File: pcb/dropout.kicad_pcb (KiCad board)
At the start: 2 copper layers, 228.6 x 94.4 mm, 64 parts, among them J1 Conn_01x04_Male, SW1 Rotary_Encoder_Switch, SW2 SW_Push, U1 ProMicro, U2 ProMicro

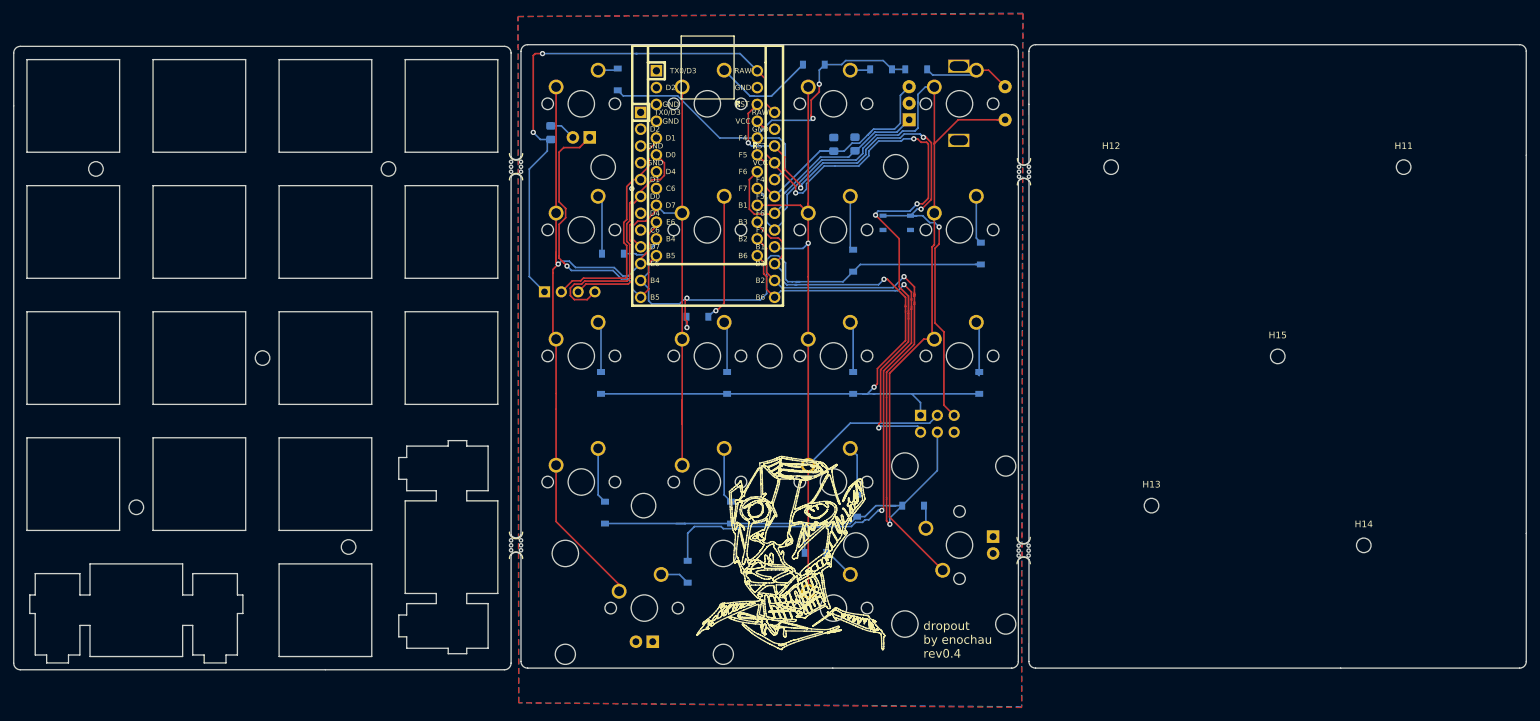
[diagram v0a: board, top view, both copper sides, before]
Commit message: updating to rev0.5
updating to rev0.5
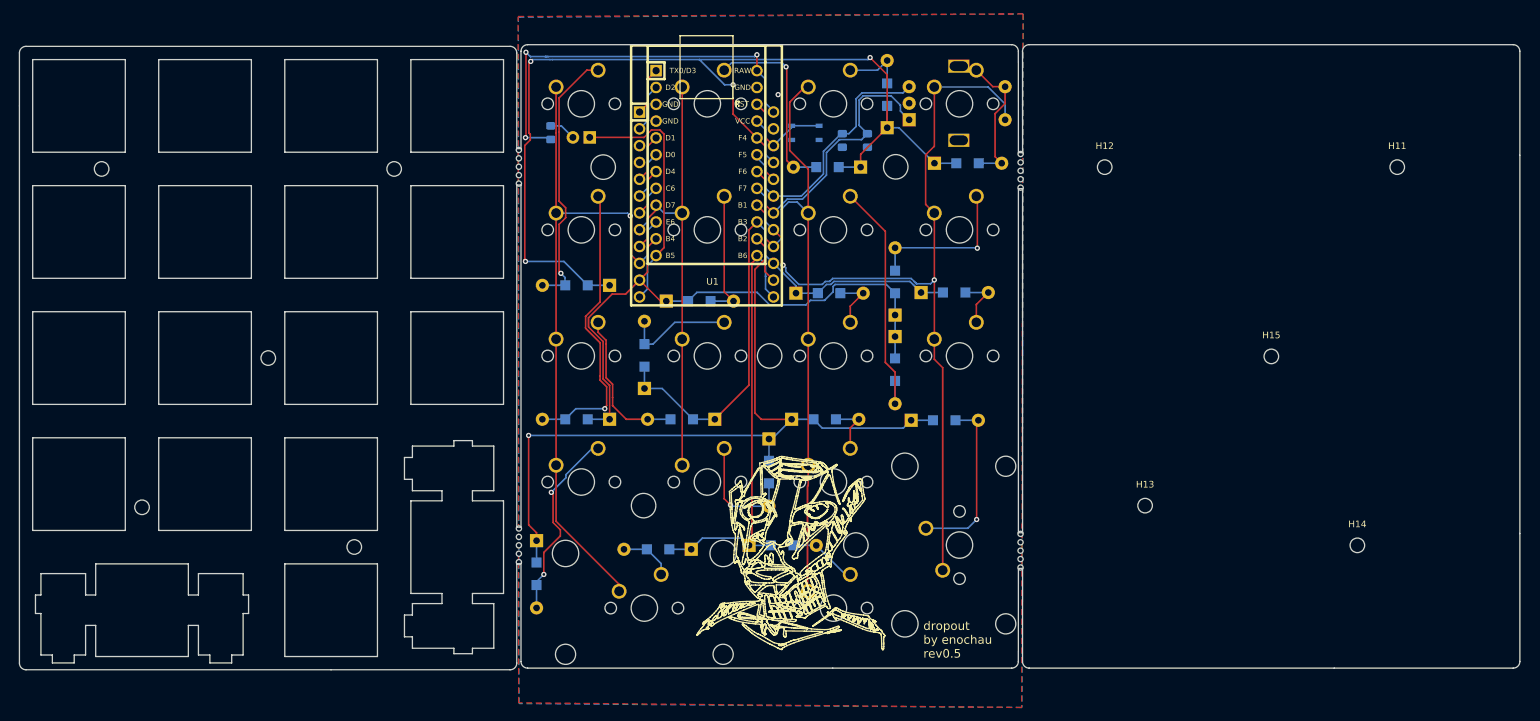
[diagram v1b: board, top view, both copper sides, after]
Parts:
- removed J-ISP1: Conn_02x03_Counter_Clockwise, Connector_PinHeader_2.54mm:PinHeader_2x03_P2.54mm_Vertical
- removed J1: Conn_01x04_Male, Connector_PinHeader_2.54mm:PinHeader_1x04_P2.54mm_Vertical
- removed U2: ProMicro, Keebio-Parts:ArduinoProMicro
- D1, D10, D11, D12, D13, D14, D15, D16, D17, D18, D2, D3, D4, D5, D6, D7, D8, D9: footprint Diode_SMD:D_SOD-123 -> footprint:Diode_TH_SOD123
- H16, H17, H18, H19: footprint Panelization:mouse-bite-2mm-slot -> Keebio-Parts:breakaway-mousebites
- K-0, K-ENT1: footprint MX_Only:MXOnly-2U-ReversedStabilizers -> MX_Only:MXOnly-2U-ReversedStabilizers-NoLED
- U1: footprint Keebio-Parts:ArduinoProMicro-Mini-USB -> promicro:ProMico_mini&micro
- moved D1 31.1 mm to (150.9, 86.9), turned to 180 degrees
- moved D2 25.0 mm to (150.9, 107.2)
- moved SW2 19.4 mm to (180.5, 63.9)
- moved D3 18.1 mm to (166.8, 107.2), turned to 180 degrees
- moved D6 17.0 mm to (188.9, 69.1)
- moved D13 16.4 mm to (178.4, 107.2), turned to 0 degrees
- moved D17 16.2 mm to (198.0, 88.0), turned to 0 degrees
- moved D12 16.1 mm to (179.1, 88.1), turned to 0 degrees
- moved D16 16.0 mm to (194.1, 91.4)
- moved D15 14.4 mm to (200.0, 68.5)
- moved D11 13.1 mm to (194.1, 94.7), turned to 270 degrees
- moved D18 12.9 mm to (196.5, 107.3)
- moved D9 12.5 mm to (175.0, 110.1), turned to 270 degrees
- moved D8 12.5 mm to (156.2, 102.5)
- moved D4 11.2 mm to (139.9, 125.5), turned to 270 degrees
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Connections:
- net RESET renamed Net-(SW2-Pad2)
- U1 pad 1: (no net) -> Net-(U1-Pad1)
- U1 pad 2: (no net) -> Net-(U1-Pad2)
- U1 pad 21: VCC -> Net-(U1-Pad21)
- U1 pad 5: SCL -> Net-(U1-Pad5)
- U1 pad 6: SDA -> Net-(U1-Pad6)
- U1 pad 7: (no net) -> Net-(U1-Pad7)
- U1 pad 8: (no net) -> Net-(U1-Pad8)
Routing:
- net VCC: track 100.0 -> 0.00 mm, vias 5 -> 0
- net ROW0: track 66.7 -> 158.8 mm, vias 2 -> 4
- net Net-(SW2-Pad2): track 95.9 -> 15.6 mm, vias 5 -> 0
- net ROW4: track 106.9 -> 68.1 mm, vias 2 -> 0
- net Net-(D1-Pad2): track 3.07 -> 40.6 mm, vias 0 -> 1
- net Net-(D2-Pad2): track 8.93 -> 44.7 mm, vias 0 -> 1
- net SCL: track 35.2 -> 0.00 mm
- net SDA: track 31.4 -> 0.00 mm
- net GND: track 29.8 -> 0.00 mm
- net Net-(D11-Pad2): track 8.37 -> 37.6 mm
- net ROW2: track 111.4 -> 86.9 mm, vias 2 -> 0
- net Net-(D18-Pad2): track 3.53 -> 26.8 mm, vias 0 -> 1
- net Net-(D4-Pad2): track 8.48 -> 29.6 mm, vias 0 -> 2
- net +5V: track 82.9 -> 62.7 mm, vias 2 -> 3
- net Net-(D16-Pad2): track 7.29 -> 23.8 mm, vias 0 -> 1
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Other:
- board size 228.6 x 94.4 mm -> 226.7 x 94.4 mm
- board text added: "dropout by enochau rev0.5"
- board text removed: "5V+"
- board text removed: "GND"
- board text removed: "RESET"
- board text removed: "SCL"
- board text removed: "SDA"
- board text removed: "VCC"
- board text removed: "dropout by enochau rev0.4"
